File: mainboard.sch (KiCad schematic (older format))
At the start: 65 parts, among them J1 Conn_01x06, J2 USB_B_Micro, J3 xf2m-2415-1a, J4 XF2M-1015-1A, J5 Conn_01x02, J6 U.FL-R-SMT-1, J7 Conn_02x02_Top_Bottom, SW1 KMR231NG LFS, U1 BMX160, U11 AP2112K-3.3, U2 MAX708RESA-T, U3 ATSAMD51J20A-M, U4 DRV8830DRC, U5 MR25H40, U6 DRV8830DRC, U8 DRV8830DRC, U9 RFM98PW-symbols

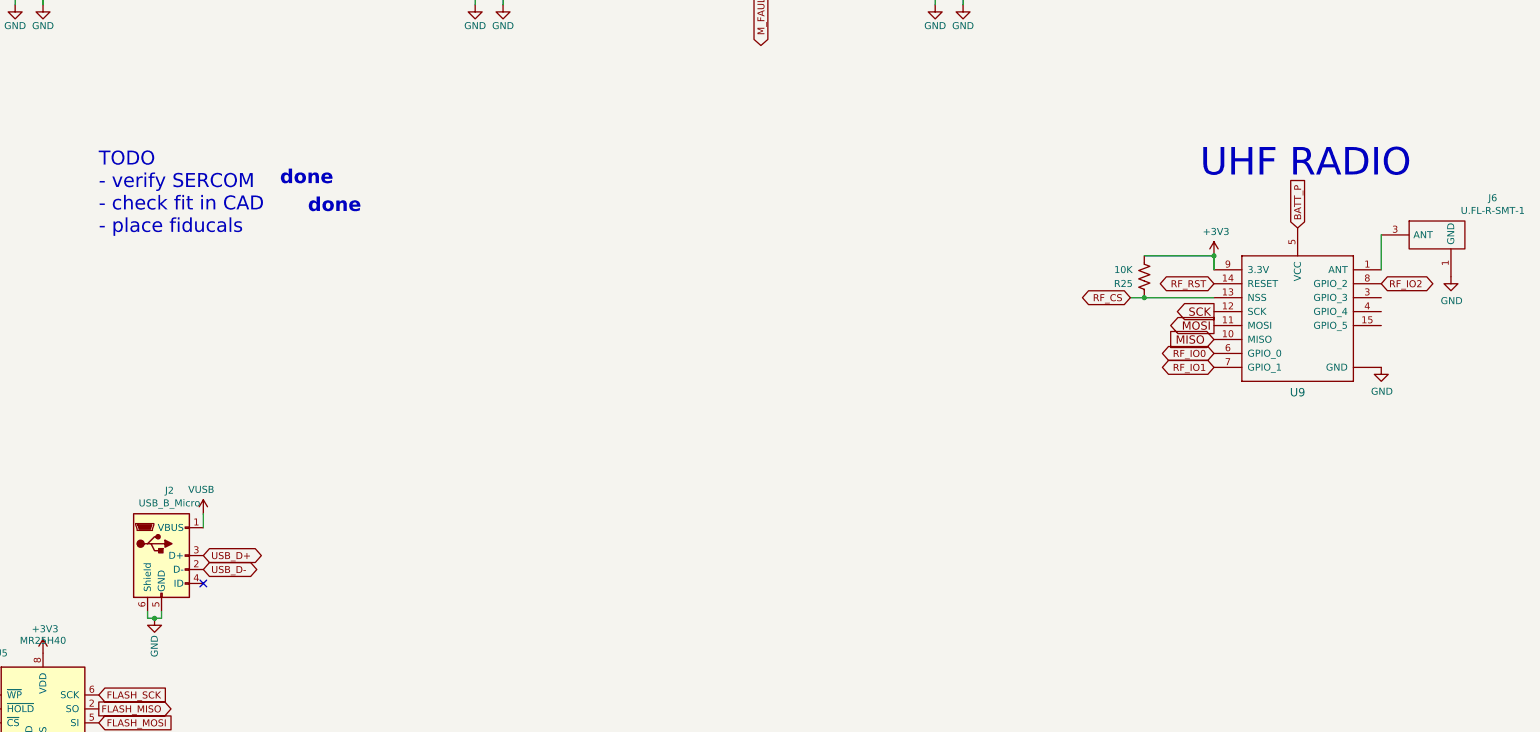
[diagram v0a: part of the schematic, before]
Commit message: roughed-in SD card
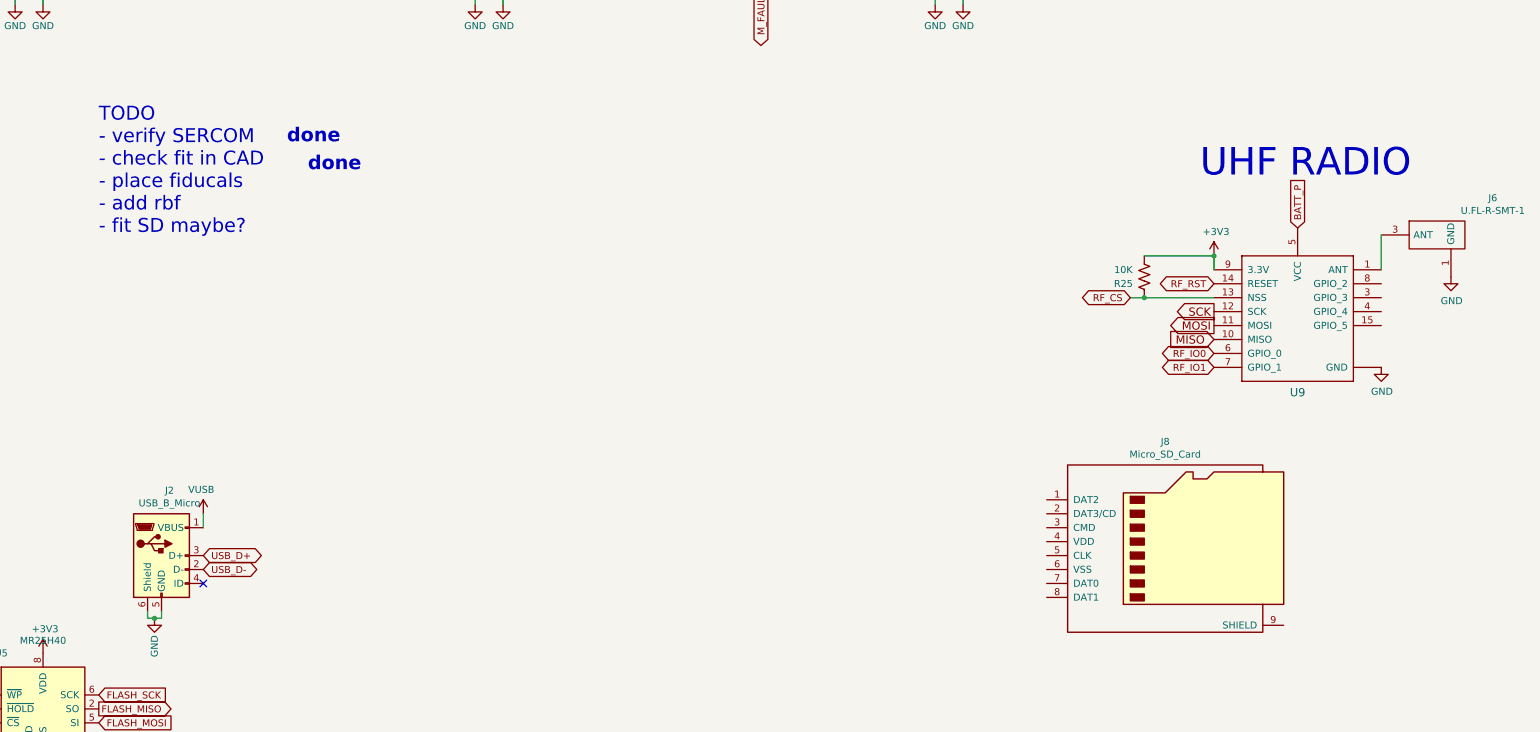
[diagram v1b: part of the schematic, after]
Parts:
- added J8: Micro_SD_Card, Connector_Card:microSD_HC_Molex_104031-0811, symbol Connector:Micro_SD_Card
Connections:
- net RF_IO2: no longer names the net of U9.8 (GPIO_2)
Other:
- note added: "TODO\n- verify SERCOM\n- check fit in CAD\n- place fiducals\n- add rbf\n- fit SD maybe?"
- note removed: "TODO\n- verify SERCOM\n- check fit in CAD\n- place fiducals"
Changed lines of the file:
@@
 Text GLabel 14400 5350 0    50   BiDi ~ 0
 RF_IO1
-Text GLabel 15600 4750 2    50   BiDi ~ 0
-RF_IO2
 Wire Wire Line
 	15600 4650 15600 4400
@@
 	0    -1   -1   0
 $EndComp
-Text Notes 6400 4400 0    100  ~ 0
-TODO\n- verify SERCOM\n- check fit in CAD\n- place fiducals
-Text Notes 7700 4050 0    100  ~ 20
+Text Notes 7750 3750 0    100  ~ 20
 done
 Text GLabel 14400 5250 0    50   BiDi ~ 0
@@
 Text GLabel 2450 7400 0    50   BiDi ~ 0
 RF_IO0
-Text Notes 7900 4250 0    100  ~ 20
+Text Notes 7900 3950 0    100  ~ 20
 done
 Wire Wire Line
@@
 	-1   0    0    -1
 $EndComp
+$Comp
+L Connector:Micro_SD_Card J8
+U 1 1 5F583739
+P 14100 6600
+F 0 "J8" H 14050 7317 50  0000 C CNN
+F 1 "Micro_SD_Card" H 14050 7226 50  0000 C CNN
+F 2 "Connector_Card:microSD_HC_Molex_104031-0811" H 15250 6900 50  0001 C CNN
+F 3 "http://katalog.we-online.de/em/datasheet/693072010801.pdf" H 14100 6600 50  0001 C CNN
+	1    14100 6600
+	1    0    0    -1
+$EndComp
+Text Notes 6400 4400 0    100  ~ 0
+TODO\n- verify SERCOM\n- check fit in CAD\n- place fiducals\n- add rbf\n- fit SD maybe?
 $EndSCHEMATC

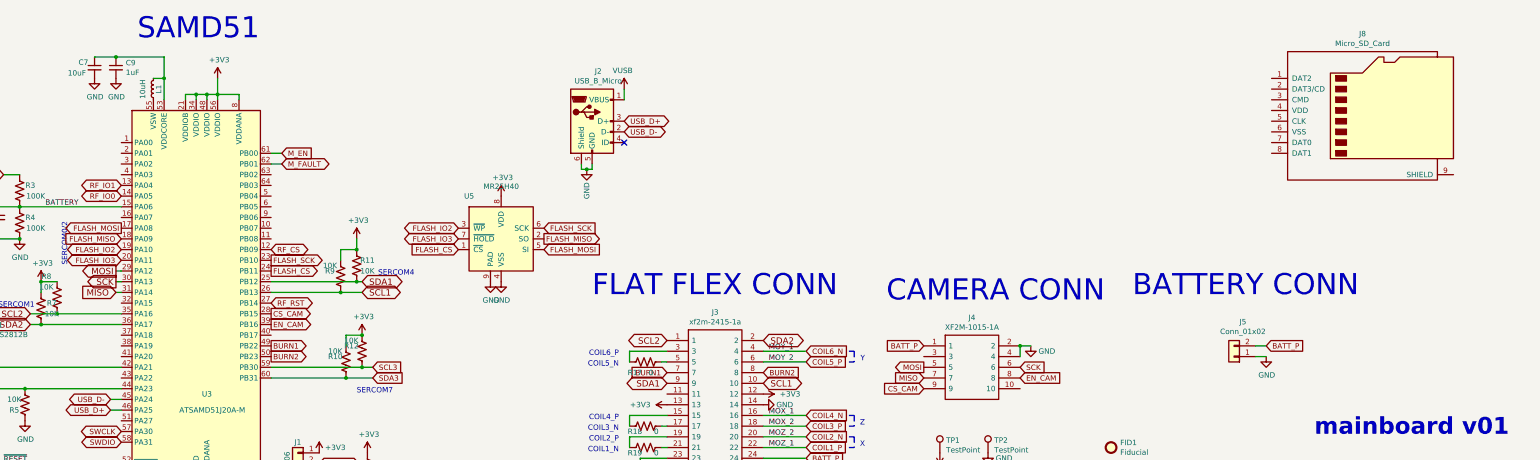
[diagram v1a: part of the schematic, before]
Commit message: routed
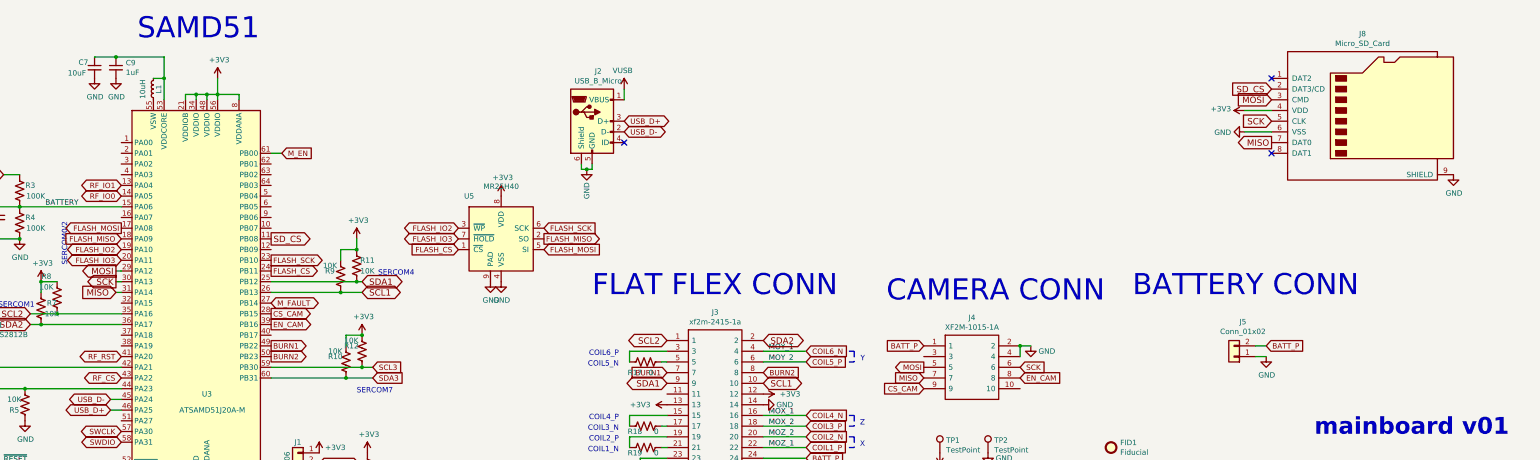
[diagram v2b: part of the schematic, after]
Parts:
- TP1, TP2: footprint TestPoint:TestPoint_Keystone_5015_Micro-Minature -> TestPoint:TestPoint_Pad_1.0x1.0mm
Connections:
- net +3V3: now also J8.4 (VDD)
- net GND: now also J8.6 (VSS), J8.9 (SHIELD)
- net MISO: now also J8.7 (DAT0)
- net MOSI: now also J8.3 (CMD)
- net M_FAULT: now also U3.27 (PB14); no longer U3.62 (PB01)
- net RF_CS: now also U3.43 (PA22); no longer U3.12 (PB09)
- net RF_RST: now also U3.41 (PA20); no longer U3.27 (PB14)
- net SCK: now also J8.5 (CLK)
- net SD_CS: now reaches U3.11 (PB08)
- net SD_CS: now also J8.2 (DAT3/CD)
- no-connect marks 8 -> 10
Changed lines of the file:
@@
 	1    0    0    -1
 $EndComp
-Text GLabel 3850 7900 2    50   BiDi ~ 0
-RF_CS
 Text GLabel 2450 7300 0    50   BiDi ~ 0
 RF_IO1
-Text GLabel 3850 8400 2    50   BiDi ~ 0
+Text GLabel 2450 8900 0    50   BiDi ~ 0
 RF_RST
 $Comp
@@
 Text GLabel 1350 7200 0    50   Input ~ 0
 BATT_P
-Text GLabel 3950 7100 2    50   BiDi ~ 0
-M_FAULT
 Text GLabel 3850 8800 2    50   Output ~ 0
 BURN1
@@
 F 0 "TP1" H 10158 9918 50  0000 L CNN
 F 1 "TestPoint" H 10158 9827 50  0000 L CNN
-F 2 "TestPoint:TestPoint_Keystone_5015_Micro-Minature" H 10300 9800 50  0001 C CNN
+F 2 "TestPoint:TestPoint_Pad_1.0x1.0mm" H 10300 9800 50  0001 C CNN
 F 3 "~" H 10300 9800 50  0001 C CNN
 	1    10100 9800
@@
 F 0 "TP2" H 10608 9918 50  0000 L CNN
 F 1 "TestPoint" H 10608 9827 50  0000 L CNN
-F 2 "TestPoint:TestPoint_Keystone_5015_Micro-Minature" H 10750 9800 50  0001 C CNN
+F 2 "TestPoint:TestPoint_Pad_1.0x1.0mm" H 10750 9800 50  0001 C CNN
 F 3 "~" H 10750 9800 50  0001 C CNN
 	1    10550 9800
@@
 Wire Wire Line
 	3850 7000 3950 7000
-Wire Wire Line
-	3850 7100 3950 7100
 Text GLabel 2450 7700 0    50   Output ~ 0
 FLASH_MOSI
@@
 Text Notes 6400 4400 0    100  ~ 0
 TODO\n- verify SERCOM\n- check fit in CAD\n- place fiducals\n- add rbf\n- fit SD maybe?
+Text GLabel 13200 6700 0    59   Input ~ 0
+SCK
+Text GLabel 13200 6500 0    59   Input ~ 0
+MOSI
+Text GLabel 13200 6900 0    59   Output ~ 0
+MISO
+Text GLabel 13200 6400 0    59   Input ~ 0
+SD_CS
+NoConn ~ 13200 7000
+NoConn ~ 13200 6300
+$Comp
+L power:GND #PWR0109
+U 1 1 5F636FAE
+P 14900 7200
+F 0 "#PWR0109" H 14900 6950 50  0001 C CNN
+F 1 "GND" H 14905 7027 50  0000 C CNN
+F 2 "" H 14900 7200 50  0001 C CNN
+F 3 "" H 14900 7200 50  0001 C CNN
+	1    14900 7200
+	1    0    0    -1
+$EndComp
+$Comp
+L power:GND #PWR0110
+U 1 1 5F637458
+P 12950 6800
+F 0 "#PWR0110" H 12950 6550 50  0001 C CNN
+F 1 "GND" V 12955 6672 50  0000 R CNN
+F 2 "" H 12950 6800 50  0001 C CNN
+F 3 "" H 12950 6800 50  0001 C CNN
+	1    12950 6800
+	0    1    1    0
+$EndComp
+Wire Wire Line
+	12950 6800 13200 6800
+$Comp
+L power:+3V3 #PWR0111
+U 1 1 5F644092
+P 12950 6600
+F 0 "#PWR0111" H 12950 6450 50  0001 C CNN
+F 1 "+3V3" V 12965 6728 50  0000 L CNN
+F 2 "" H 12950 6600 50  0001 C CNN
+F 3 "" H 12950 6600 50  0001 C CNN
+	1    12950 6600
+	0    -1   -1   0
+$EndComp
+Wire Wire Line
+	12950 6600 13200 6600
+Text GLabel 3850 7800 2    59   Output ~ 0
+SD_CS
+Text GLabel 3850 8400 2    50   BiDi ~ 0
+M_FAULT
+Text GLabel 2450 9100 0    50   BiDi ~ 0
+RF_CS
 $EndSCHEMATC
